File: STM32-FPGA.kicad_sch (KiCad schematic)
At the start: 18 parts, among them J1 USB4105-GF-A-120, J4 Conn_01x04, J5 Conn_01x05, U4 USBLC6-2SC6

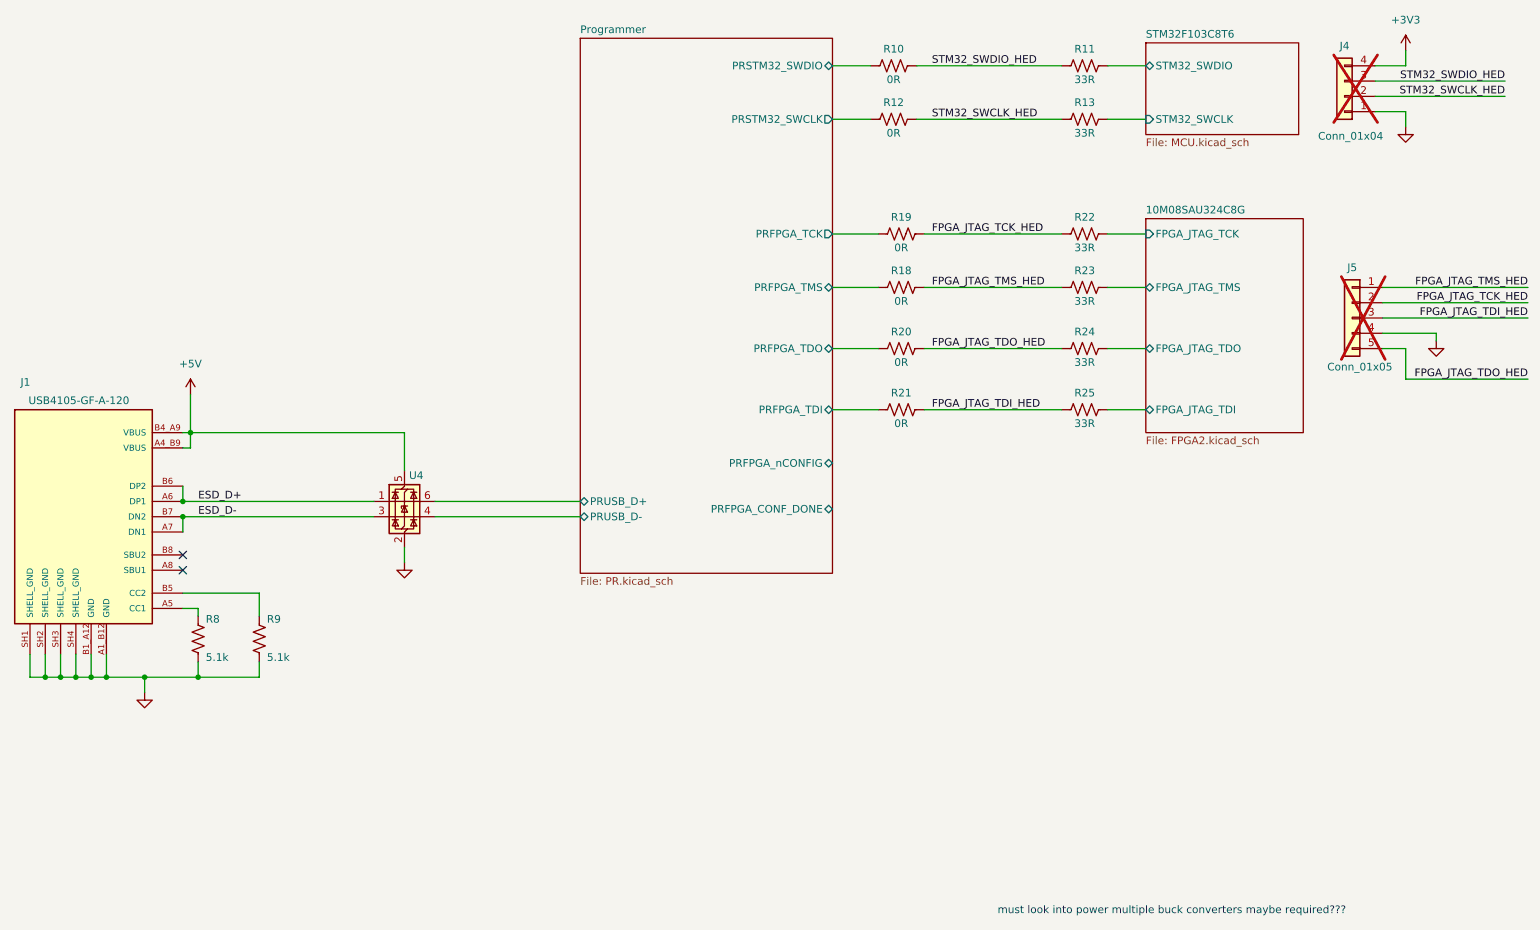
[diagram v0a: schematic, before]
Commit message: power supply
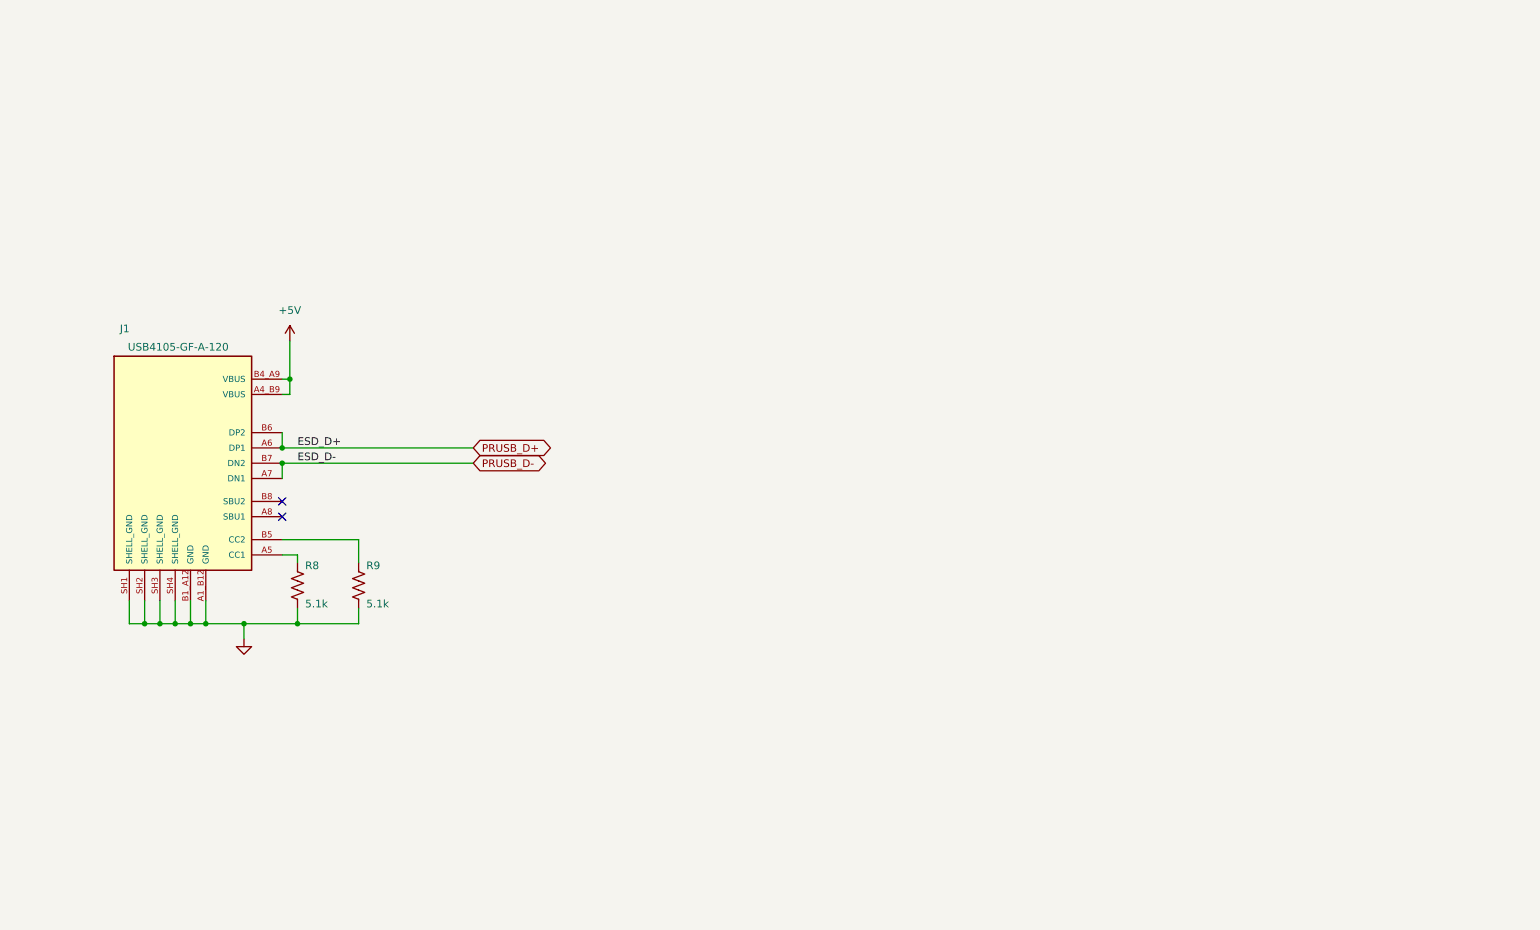
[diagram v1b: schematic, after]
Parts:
- removed J4: Conn_01x04, symbol Connector_Generic:Conn_01x04
- removed J5: Conn_01x05, symbol Connector_Generic:Conn_01x05
- removed R10, R12, R18, R19, R20, R21: 0R, symbol Device:R_US
- removed R11, R13, R22, R23, R24, R25: 33R, symbol Device:R_US
- removed U4: USBLC6-2SC6, Package_TO_SOT_SMD:SOT-23-6, symbol Power_Protection:USBLC6-2SC6
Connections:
- net ESD_D+ renamed PRUSB_D+
- net ESD_D- renamed PRUSB_D-
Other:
- removed sheet 10M08SAU324C8G
- removed sheet Programmer
- removed sheet STM32F103C8T6
- note removed: "must look into power multiple buck converters maybe required???"
- moved on the sheet: J1, R8, R9
